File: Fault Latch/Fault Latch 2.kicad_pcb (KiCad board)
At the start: 2 copper layers, 85 x 85 mm, 116 parts, among them J1 1053141312, J3 1053131202, J4 1053131202, J5 1053131202, K3 Fujitsu_FTR-LYCA005x, K5 Fujitsu_FTR-LYCA005x, K6 Fujitsu_FTR-LYCA005x, Q101 Q_NPN_BEC, Q102 Q_NPN_BEC, Q103 Q_NPN_BEC, Q104 Q_NPN_BEC, Q105 Q_NMOS_GSD, Q106 Q_NMOS_GSD, Q110 Q_NPN_BEC, Q111 Q_NPN_BEC, Q112 Q_NMOS_GSD, Q113 Q_NMOS_GSD, Q114 Q_NMOS_GSD, Q115 Q_NMOS_GSD, Q117 Q_NMOS_GSD, Q118 Q_NMOS_GSD, Q119 Q_NMOS_GSD, Q120 Q_NMOS_GSD, Q121 Q_NMOS_GSD, Q122 Q_NMOS_GSD, Q123 Q_NMOS_GSD, Q124 Q_NMOS_GSD, Q125 Q_NMOS_GSD, SW101 SW_Omron_B3FS, SW102 SW_Omron_B3FS, SW103 SW_Omron_B3FS, U1 74LS279, U104 74AHC1G00, U109 74AHC1G00, U112 74AHC1G00, U117 74AHC1G00, U118 LM555xM, U2 LM1117DT-5.0, U7 SN74AHC1G08DBVR, U8 SN74AHC1G08DBVR

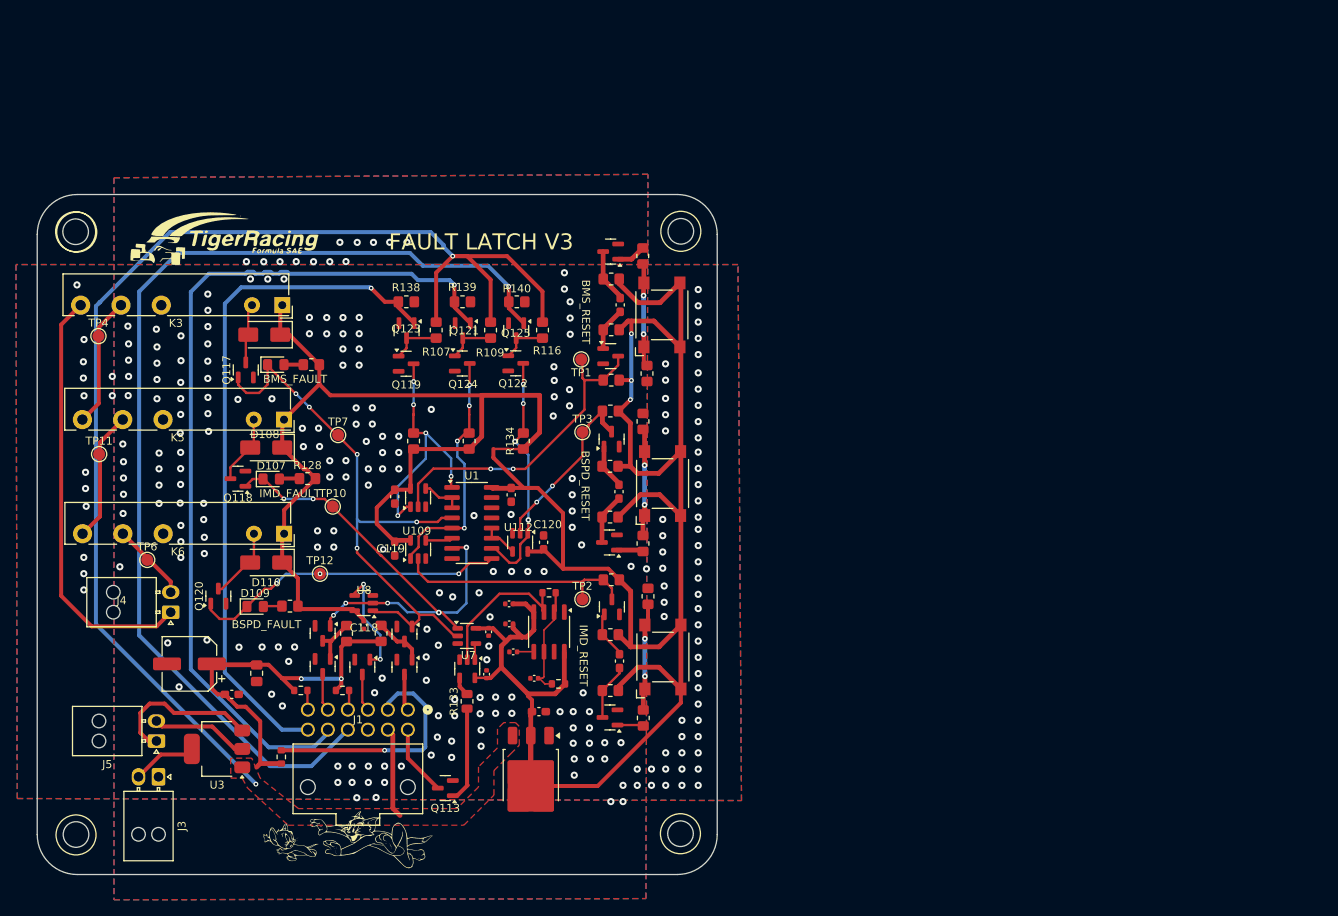
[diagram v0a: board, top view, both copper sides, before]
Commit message: Bom + Schematic Redone V3.2
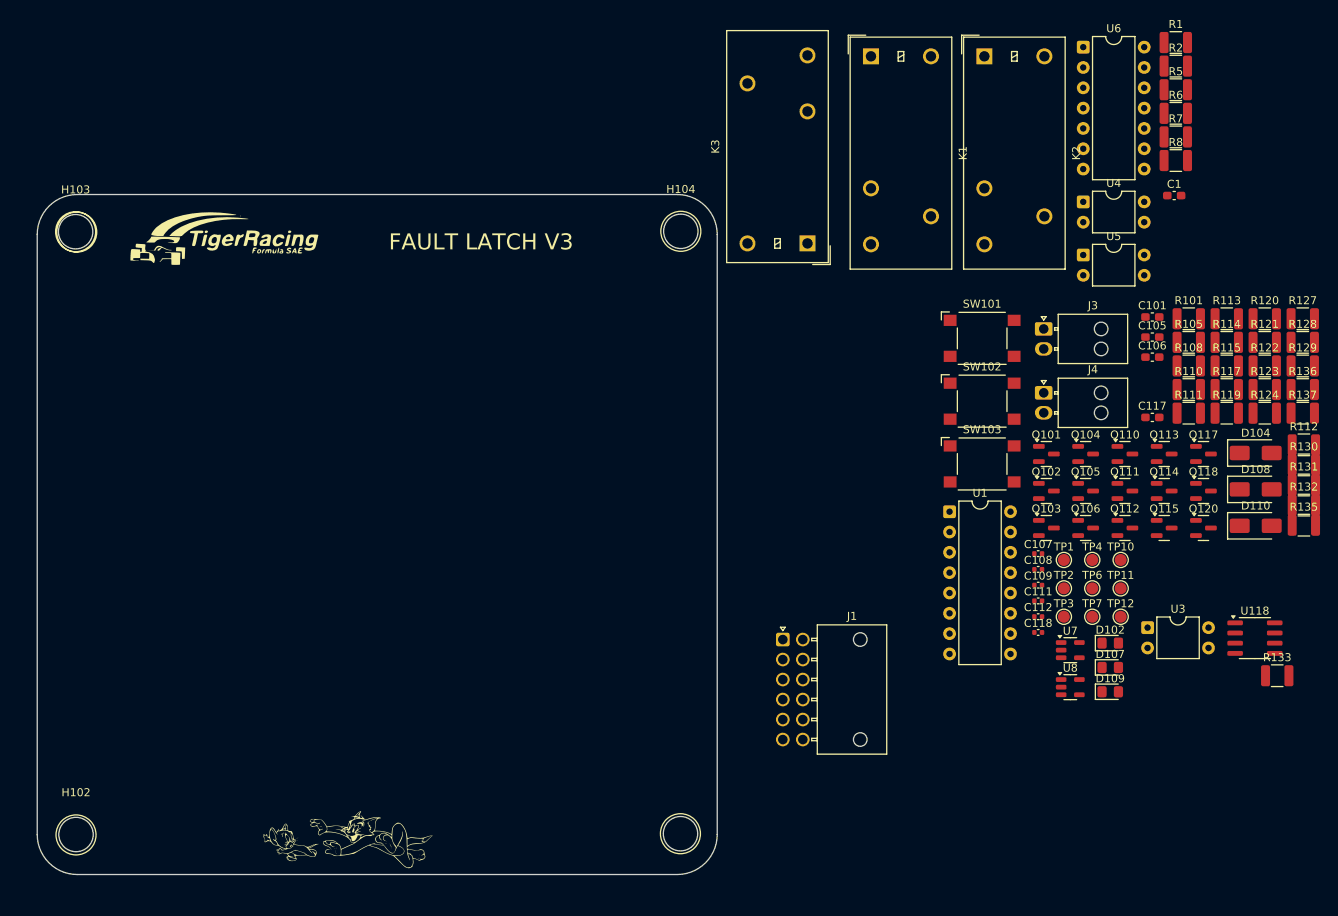
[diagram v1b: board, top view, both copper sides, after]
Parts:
- removed C102, C116, C119, C120: 100n, Capacitor_SMD:C_0603_1608Metric_Pad1.08x0.95mm_HandSolder
- removed C110: 0.1u, Capacitor_SMD:C_0402_1005Metric
- removed C113: 47u, Capacitor_SMD:CP_Elec_6.3x5.4
- removed C114: 1u, Capacitor_SMD:C_0805_2012Metric_Pad1.18x1.45mm_HandSolder
- removed C115: 0.33u, Capacitor_SMD:C_0603_1608Metric_Pad1.08x0.95mm_HandSolder
- removed J5: 1053131202, Connector_Molex:Molex_Nano-Fit_105313-xx02_1x02_P2.50mm_Horizontal
- removed K5, K6: Fujitsu_FTR-LYCA005x, Relay_THT:Relay_SPDT_Fujitsu_FTR-LYCA005x_FormC_Vertical
- removed Q119, Q121, Q122, Q123, Q124, Q125: Q_NMOS_GSD, Package_TO_SOT_SMD:SOT-23
- removed R106, R107, R109, R116, R126, R134: 1k, Resistor_SMD:R_0805_2012Metric_Pad1.20x1.40mm_HandSolder
- removed R138, R139, R140: 10k, Resistor_SMD:R_0805_2012Metric_Pad1.20x1.40mm_HandSolder
- removed U104, U109, U112, U117: 74AHC1G00, Package_TO_SOT_SMD:SOT-23-5
- removed U2: LM1117DT-5.0, Package_TO_SOT_SMD:TO-252-3_TabPin2
- added C1: 100n, Capacitor_SMD:C_0603_1608Metric_Pad1.08x0.95mm_HandSolder, F.Cu at (211.4, 44.5)
- added K1: Relay_SPDT_Omron_G2RL-1, Relay_THT:Relay_SPDT_Omron_G2RL-1, F.Cu at (173.5, 27.1)
- added K2: Relay_SPDT_Omron_G2RL-1, Relay_THT:Relay_SPDT_Omron_G2RL-1, F.Cu at (187.7, 27.1)
- added R1: 1k, Resistor_SMD:R_1210_3225Metric, F.Cu at (211.6, 25.4)
- added R2: 10k, Resistor_SMD:R_1210_3225Metric, F.Cu at (211.6, 28.3)
- added R5: 10k, Resistor_SMD:R_1210_3225Metric, F.Cu at (211.6, 31.3)
- added R6: 1k, Resistor_SMD:R_1210_3225Metric, F.Cu at (211.6, 34.2)
- added R7: 1k, Resistor_SMD:R_1210_3225Metric, F.Cu at (211.6, 37.2)
- added R8: 10k, Resistor_SMD:R_1210_3225Metric, F.Cu at (211.6, 40.1)
- added U4: SFH617A-1, Package_DIP:DIP-4_W7.62mm, F.Cu at (200.0, 45.3)
- added U5: SFH617A-1, Package_DIP:DIP-4_W7.62mm, F.Cu at (200.0, 51.9)
- added U6: 74HCT00, Package_DIP:DIP-14_W7.62mm, F.Cu at (200.0, 26.0)
- H101, H102, H103, H104: footprint MountingHole:MountingHole_3.2mm_M3 -> MountingHole:MountingHole_4.3mm_M4
- J1: footprint footprints:CONN_SD-105314-100_12_MOL -> Connector_Molex:Molex_Nano-Fit_105314-xx12_2x06_P2.50mm_Horizontal
- K3: value Fujitsu_FTR-LYCA005x -> Relay_SPDT_Omron_G2RL-1; footprint Relay_THT:Relay_SPDT_Fujitsu_FTR-LYCA005x_FormC_Vertical -> Relay_THT:Relay_SPDT_Omron_G2RL-1
- R101, R105, R108, R110, R111, R113, R114, R115, R117, R119, R120, R121, R122, R123, R124, R127, R128, R129, R136, R137: footprint Resistor_SMD:R_0805_2012Metric_Pad1.20x1.40mm_HandSolder -> Resistor_SMD:R_1210_3225Metric
- R112, R130, R131, R132, R135: footprint Resistor_SMD:R_0603_1608Metric -> Resistor_SMD:R_1210_3225Metric
- R133: footprint Resistor_SMD:R_0805_2012Metric -> Resistor_SMD:R_1210_3225Metric
- TP1: value TestPoint_BMS -> TestPoint
- TP10, TP12, TP7: value TestPoint_SR_BMS -> TestPoint
- TP11: value TestPoint_IMD_Shutdown -> TestPoint
- TP2: value TestPoint_IMD -> TestPoint
- TP3: value TestPoint_BSPD -> TestPoint
- TP4: value TestPoint_BMS_Shutdown -> TestPoint
- TP6: value TestPoint_BSPD_Shutdown -> TestPoint
- U1: footprint Package_SO:SOIC-16_3.9x9.9mm_P1.27mm -> Package_DIP:DIP-16_W7.62mm
- U3: value ~ -> SFH617A-1; footprint Package_TO_SOT_SMD:SOT-223 -> Package_DIP:DIP-4_W7.62mm
- moved R135 131.1 mm to (227.6, 85.7), turned to 0 degrees
- moved R112 129.1 mm to (227.6, 75.7)
- moved R137 128.9 mm to (227.5, 71.7)
- moved TP11 128.8 mm to (204.7, 93.6)
- moved TP4 127.3 mm to (201.2, 90.1)
- moved R128 125.6 mm to (227.5, 62.9)
- moved D104 124.8 mm to (221.6, 76.7), turned to 0 degrees
- moved J3 124.0 mm to (195.1, 61.2), turned to 0 degrees
- moved D108 123.8 mm to (221.6, 81.2), turned to 0 degrees
- moved D110 123.8 mm to (221.6, 85.8), turned to 0 degrees
- moved Q120 123.4 mm to (215.1, 86.1), turned to 0 degrees
- moved R130 123.4 mm to (227.6, 78.2), turned to 0 degrees
- moved Q118 120.7 mm to (215.1, 81.4), turned to 0 degrees
- moved R121 120.4 mm to (222.7, 62.9), turned to 0 degrees
- moved Q117 120.2 mm to (215.1, 76.8), turned to 0 degrees
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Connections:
- D104 pad 1: +5V -> +12V
- D108 pad 1: +5V -> +12V
- D110 pad 1: +5V -> +12V
- K3 pad 11: Net-(K3-Pad11) -> /Shutdown Circuit Out
- K3 pad 12: GND -> unconnected-(K3-Pad12)
- K3 pad 14: /Shutdown Circuit In -> Net-(K2-Pad11)
- K3 pad A1: +5V -> +12V
- K3 pad A2: Net-(D104-A) -> Net-(D110-A)
- TP11 pad 1: Net-(K5-Pad11) -> Net-(K2-Pad11)
- TP4 pad 1: Net-(K3-Pad11) -> Net-(K1-Pad11)
- U3 pad 2: /Load Switch - -> /IMD_HV
- U3 pad 3: /Load Switch + -> GND
- U3 pad 4: /LVB -> Net-(R1-Pad2)
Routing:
- net +5V: track 380.7 -> 0.00 mm, vias 3 -> 0
- net +12V: track 216.1 -> 0.00 mm, vias 4 -> 0
- net /BSPD_HV: track 133.0 -> 0.00 mm, vias 1 -> 0
- net /IMD_HV: track 109.7 -> 0.00 mm, vias 1 -> 0
- net /NBMS_HV: track 86.2 -> 0.00 mm, vias 1 -> 0
- net /BMS_SR: track 72.4 -> 0.00 mm, vias 5 -> 0
- net /IMD_SR: track 63.0 -> 0.00 mm, vias 7 -> 0
- net /Shutdown Circuit In: track 53.4 -> 0.00 mm
- net /NRESET_BMS: track 39.9 -> 0.00 mm, vias 2 -> 0
- net Net-(D109-K): track 39.5 -> 0.00 mm, vias 3 -> 0
- net /NBMS_LV: track 32.3 -> 0.00 mm, vias 5 -> 0
- net /NRESET_IMD: track 30.8 -> 0.00 mm
- net /NIMD_LV: track 30.3 -> 0.00 mm, vias 4 -> 0
- net /BMS Light In: track 30.0 -> 0.00 mm, vias 1 -> 0
- net /NBPSD_LV: track 29.5 -> 0.00 mm, vias 4 -> 0
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- removed copper zone on F.Cu, net +12V
- removed copper zone on B.Cu, net GND
- removed copper zone on F.Cu, net GND
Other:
- board text removed: "BMS_FAULT"
- board text removed: "BMS_RESET"
- board text removed: "BSPD_FAULT"
- board text removed: "BSPD_RESET"
- board text removed: "IMD_FAULT"
- board text removed: "IMD_RESET"
